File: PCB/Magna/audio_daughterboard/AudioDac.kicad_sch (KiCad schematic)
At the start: 44 parts, among them U401 NE5532, U403 PCM1789

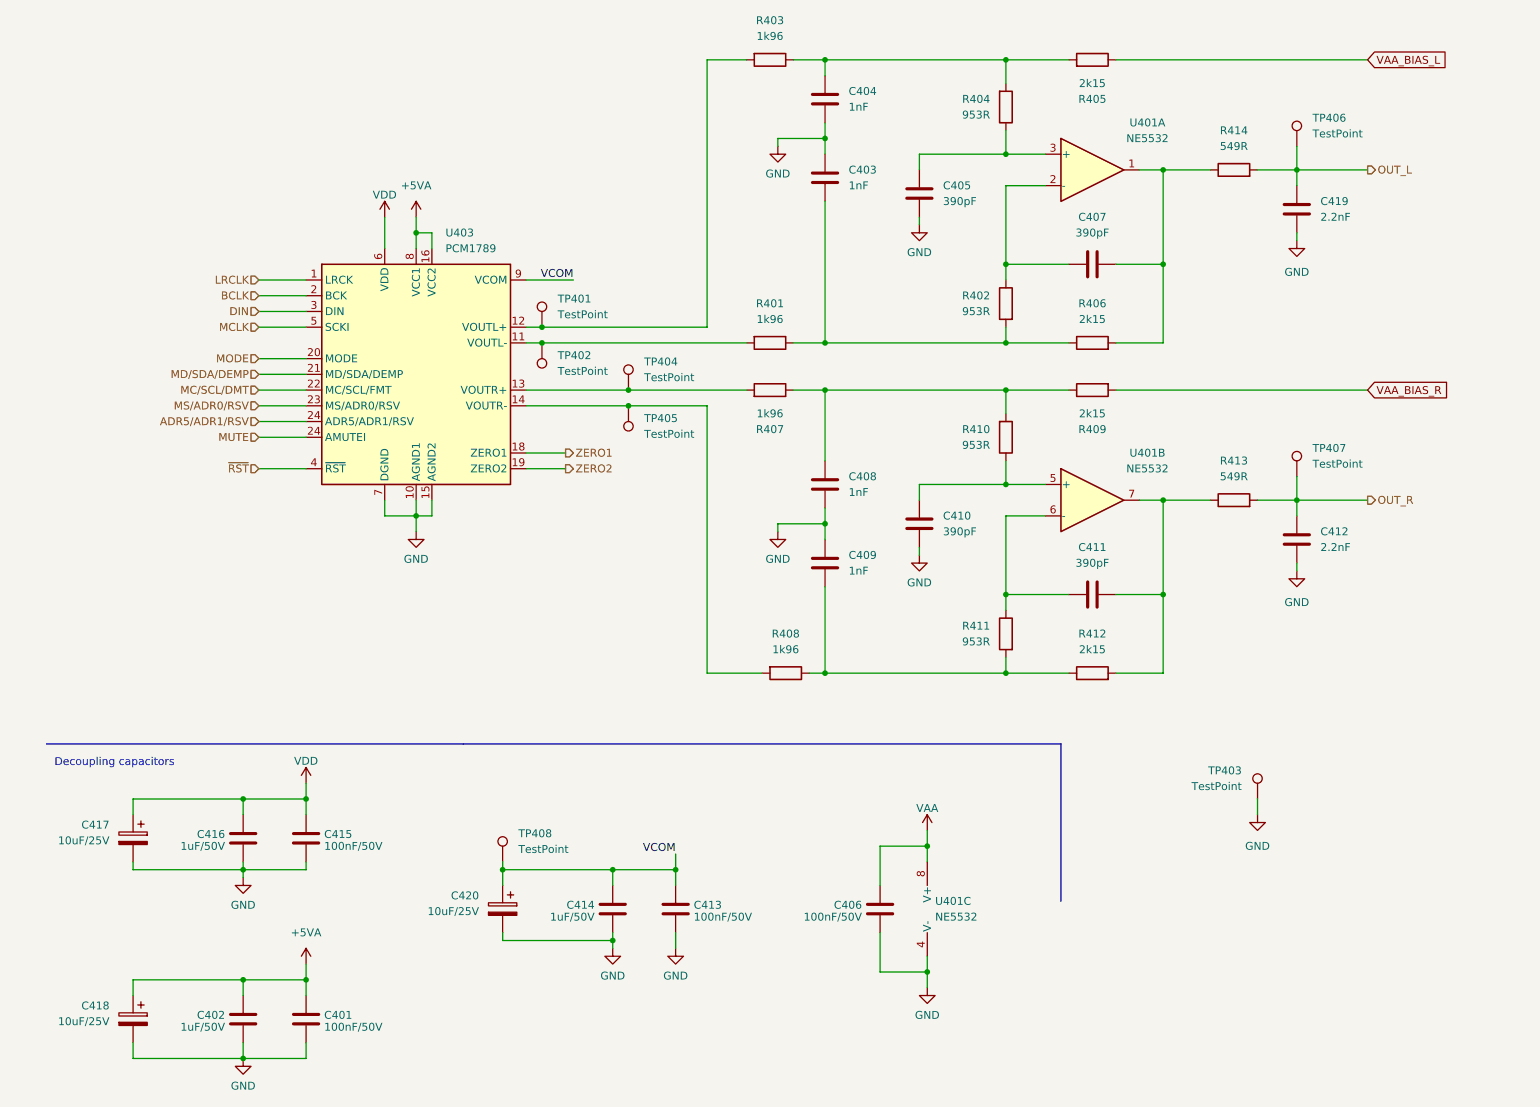
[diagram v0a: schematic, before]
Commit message: Some updates to PCB
Honestly I cannot remember whats changed
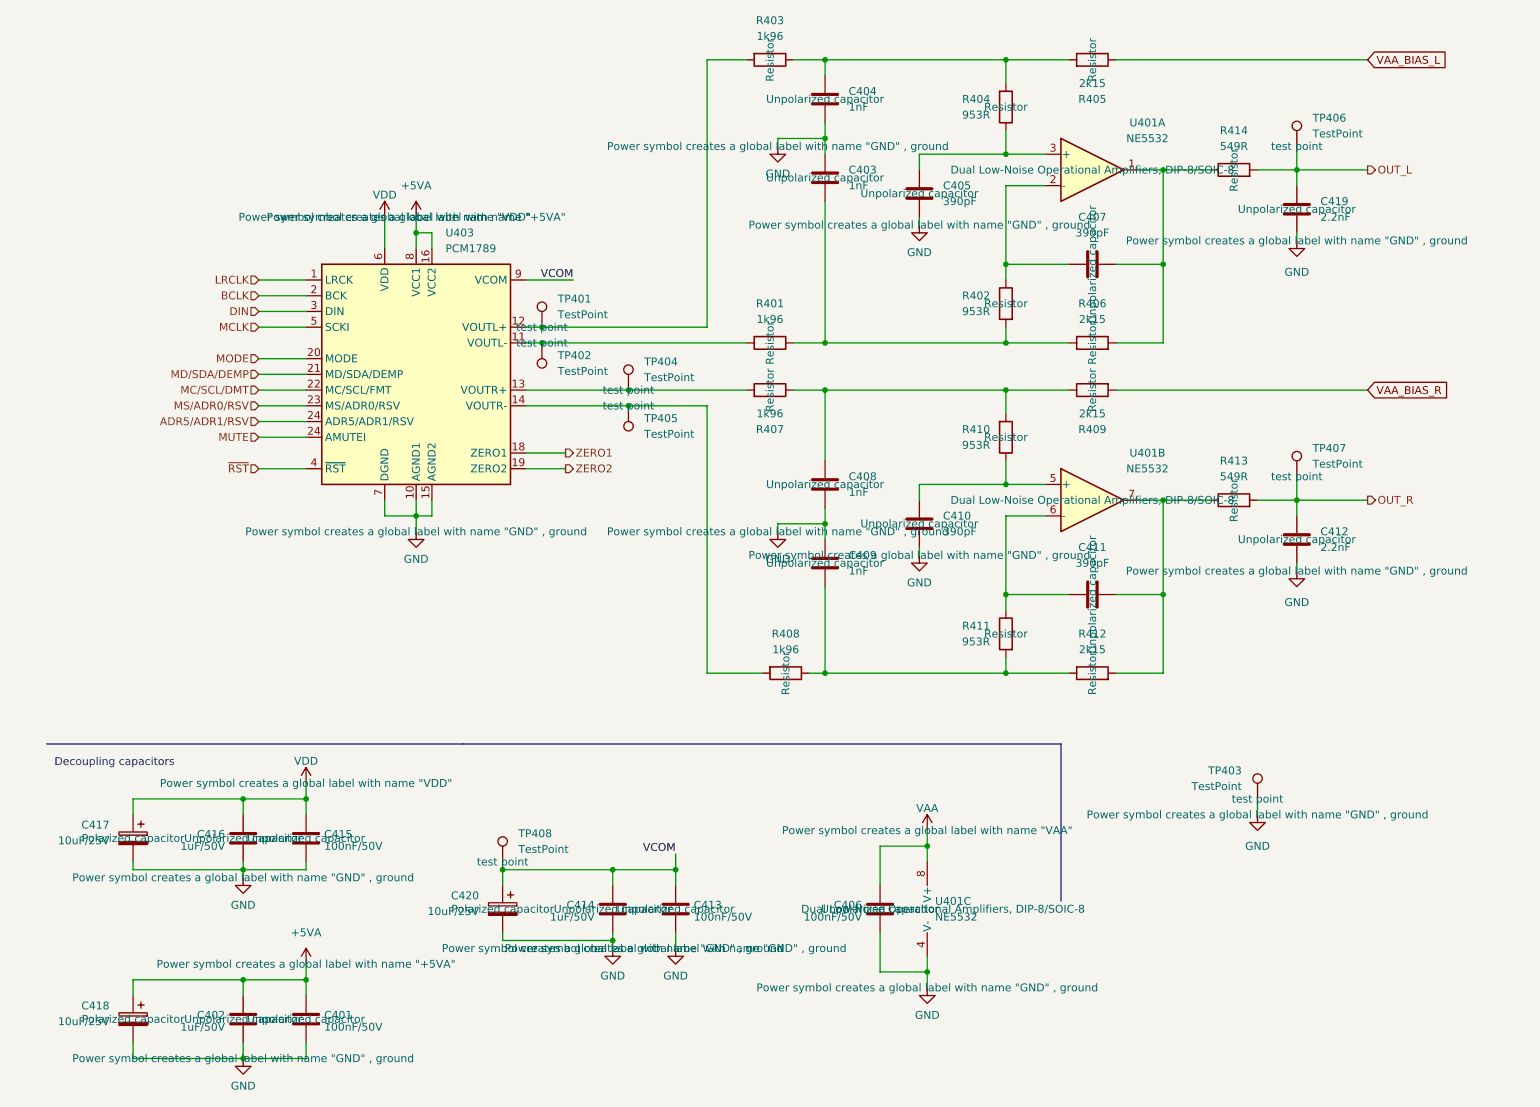
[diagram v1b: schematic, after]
